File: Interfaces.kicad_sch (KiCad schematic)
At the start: 15 parts, among them J14 I2C1_Headers, J15 SPI1_Headers, J16 General_Pin_Header, J3 LPUART1_Headers, J8 Debug_Pins

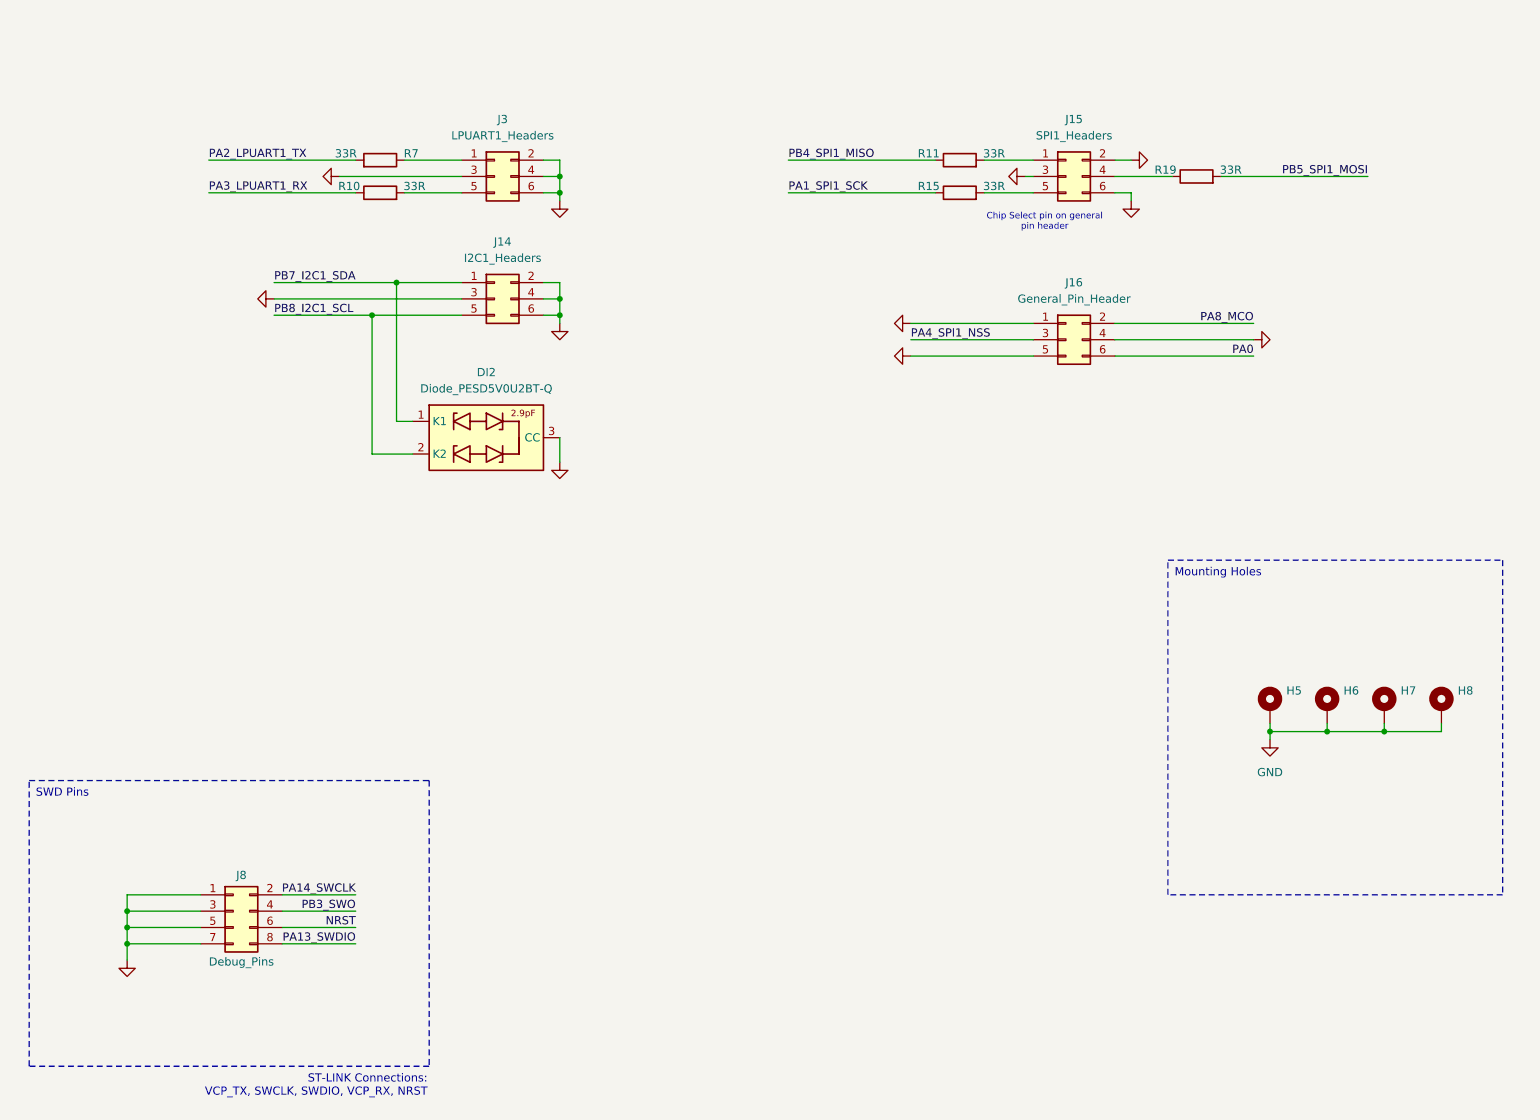
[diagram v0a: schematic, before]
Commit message: Update
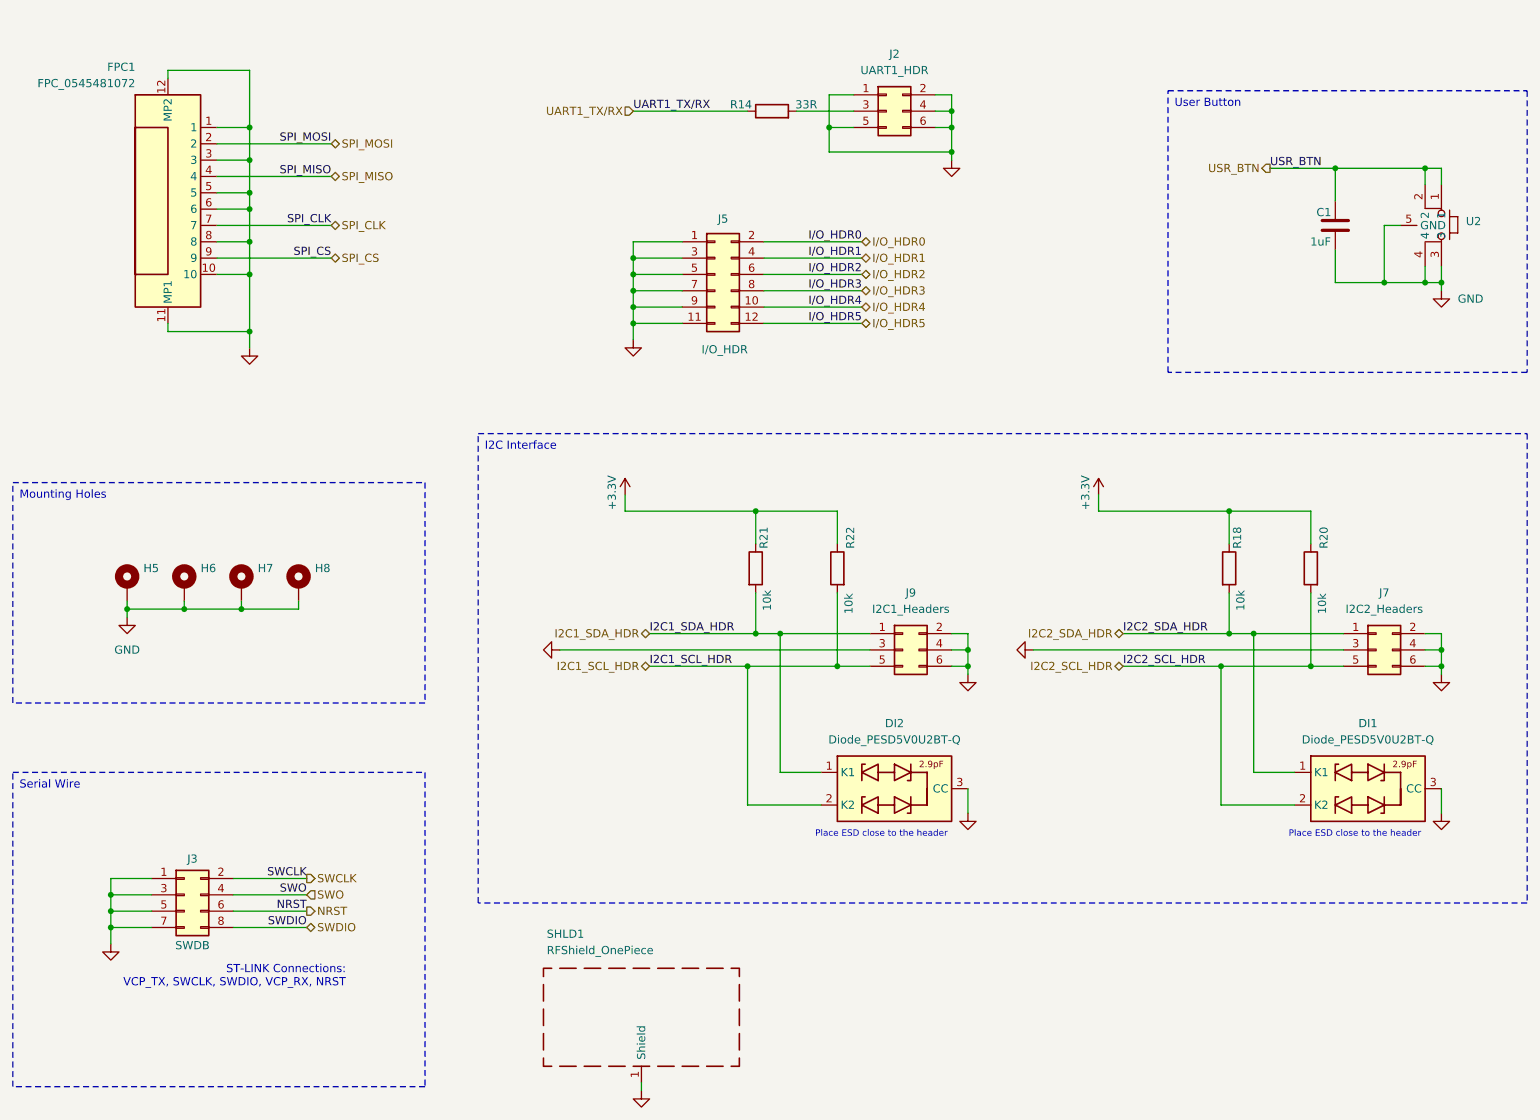
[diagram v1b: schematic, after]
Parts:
- removed J14: I2C1_Headers, Connector_PinHeader_2.54mm:PinHeader_2x03_P2.54mm_Horizontal, symbol Connector_Generic:Conn_02x03_Odd_Even
- removed J15: SPI1_Headers, Connector_PinHeader_2.54mm:PinHeader_2x03_P2.54mm_Horizontal, symbol Connector_Generic:Conn_02x03_Odd_Even
- removed J16: General_Pin_Header, Connector_PinHeader_2.54mm:PinHeader_2x03_P2.54mm_Horizontal, symbol Connector_Generic:Conn_02x03_Odd_Even
- removed J3: LPUART1_Headers, Connector_PinHeader_2.54mm:PinHeader_2x03_P2.54mm_Horizontal, symbol Connector_Generic:Conn_02x03_Odd_Even
- removed J8: Debug_Pins, Connector_PinHeader_2.54mm:PinHeader_2x04_P2.54mm_Horizontal, symbol Connector_Generic:Conn_02x04_Odd_Even
- removed R10, R11, R15, R19, R7: 33R, Resistor_SMD:R_0805_2012Metric, symbol Device:R
- added C1: 1uF, Capacitor_SMD:C_0805_2012Metric, symbol Device:C
- added DI1: Diode_PESD5V0U2BT-Q, Package_TO_SOT_SMD:SOT-23, symbol Personal_Projects:Diode_PESD5V0U2BT-Q
- added FPC1: FPC_0545481072, Personal_Project:FPC_0545481072, symbol Personal_Projects:FPC_0545481072
- added J2: UART1_HDR, Connector_PinHeader_2.54mm:PinHeader_2x03_P2.54mm_Horizontal, symbol Connector_Generic:Conn_02x03_Odd_Even
- added J3: SWDB, Connector_PinHeader_2.54mm:PinHeader_2x04_P2.54mm_Horizontal, symbol Connector_Generic:Conn_02x04_Odd_Even
- added J5: I/O_HDR, symbol Connector_Generic:Conn_02x06_Odd_Even
- added J7: I2C2_Headers, Connector_PinHeader_2.54mm:PinHeader_2x03_P2.54mm_Horizontal, symbol Connector_Generic:Conn_02x03_Odd_Even
- added J9: I2C1_Headers, Connector_PinHeader_2.54mm:PinHeader_2x03_P2.54mm_Horizontal, symbol Connector_Generic:Conn_02x03_Odd_Even
- added R14: 33R, Resistor_SMD:R_0805_2012Metric, symbol Device:R
- added R18, R20, R21, R22: 10k, Resistor_SMD:R_0805_2012Metric, symbol Device:R
- added SHLD1: RFShield_OnePiece, Personal_Project:RF_Shield_MS631-10F, symbol Device:RFShield_OnePiece
- added U2: ~, Personal_Project:Button_KMR231GLFS, symbol Personal_Projects:Button_KMR231GLFS
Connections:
- net GND: now also C1.1, DI1.3 (CC), FPC1.1, FPC1.10, FPC1.11 (MP1), FPC1.12 (MP2), FPC1.3, FPC1.5, FPC1.6, FPC1.8, J2.1 (Pin_1), J2.2 (Pin_2), J2.4 (Pin_4), J2.5 (Pin_5), J2.6 (Pin_6), J3.1 (Pin_1), J3.3 (Pin_3), J3.5 (Pin_5), J3.7 (Pin_7), J5.1 (Pin_1), J5.11 (Pin_11), J5.3 (Pin_3), J5.5 (Pin_5), J5.7 (Pin_7), J5.9 (Pin_9), J7.2 (Pin_2), J7.3 (Pin_3), J7.4 (Pin_4), J7.6 (Pin_6), J9.2 (Pin_2), J9.3 (Pin_3), J9.4 (Pin_4), J9.6 (Pin_6), SHLD1.1 (Shield), U2.3, U2.4, U2.5 (GND)
- net NRST: now also J3.6 (Pin_6)
- net PB7_I2C1_SDA renamed I2C1_SDA_HDR
- net I2C1_SDA_HDR: now also J9.1 (Pin_1), R21.2
- net PB8_I2C1_SCL renamed I2C1_SCL_HDR
- net I2C1_SCL_HDR: now also J9.5 (Pin_5), R22.2
- new net: J2.3 (Pin_3), R14.2
- new net +3.3V: R18.1, R20.1, R21.1, R22.1
- new net I2C2_SCL_HDR: DI1.2 (K2), J7.5 (Pin_5), R20.2
- new net I2C2_SDA_HDR: DI1.1 (K1), J7.1 (Pin_1), R18.2
- new net I/O_HDR0: J5.2 (Pin_2)
- new net I/O_HDR1: J5.4 (Pin_4)
- new net I/O_HDR2: J5.6 (Pin_6)
- new net I/O_HDR3: J5.8 (Pin_8)
- new net I/O_HDR4: J5.10 (Pin_10)
- new net I/O_HDR5: J5.12 (Pin_12)
- new net SPI_CLK: FPC1.7
- new net SPI_CS: FPC1.9
- new net SPI_MISO: FPC1.4
- new net SPI_MOSI: FPC1.2
- new net SWCLK: J3.2 (Pin_2)
- new net SWDIO: J3.8 (Pin_8)
- new net SWO: J3.4 (Pin_4)
- new net UART1_TX/RX: R14.1
- new net USR_BTN: C1.2, U2.1, U2.2
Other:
- note added: "Place ESD close to the header"
- note removed: "Chip Select pin on general pin header"
- moved on the sheet: H5, H6, H7, H8

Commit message: Update
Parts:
- J5: footprint (none) -> Connector_PinHeader_2.54mm:PinHeader_2x06_P2.54mm_Vertical
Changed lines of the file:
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@@
 			)
 		)
-		(property "Footprint" ""
+		(property "Footprint" "Connector_PinHeader_2.54mm:PinHeader_2x06_P2.54mm_Vertical"
 			(at 133.35 66.04 0)
 			(effects

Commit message: Update
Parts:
- J5: footprint Connector_PinHeader_2.54mm:PinHeader_2x06_P2.54mm_Vertical -> Connector_PinHeader_2.54mm:PinHeader_2x06_P2.54mm_Horizontal
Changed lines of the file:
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@@
 			)
 		)
-		(property "Footprint" "Connector_PinHeader_2.54mm:PinHeader_2x06_P2.54mm_Vertical"
+		(property "Footprint" "Connector_PinHeader_2.54mm:PinHeader_2x06_P2.54mm_Horizontal"
 			(at 133.35 66.04 0)
 			(effects

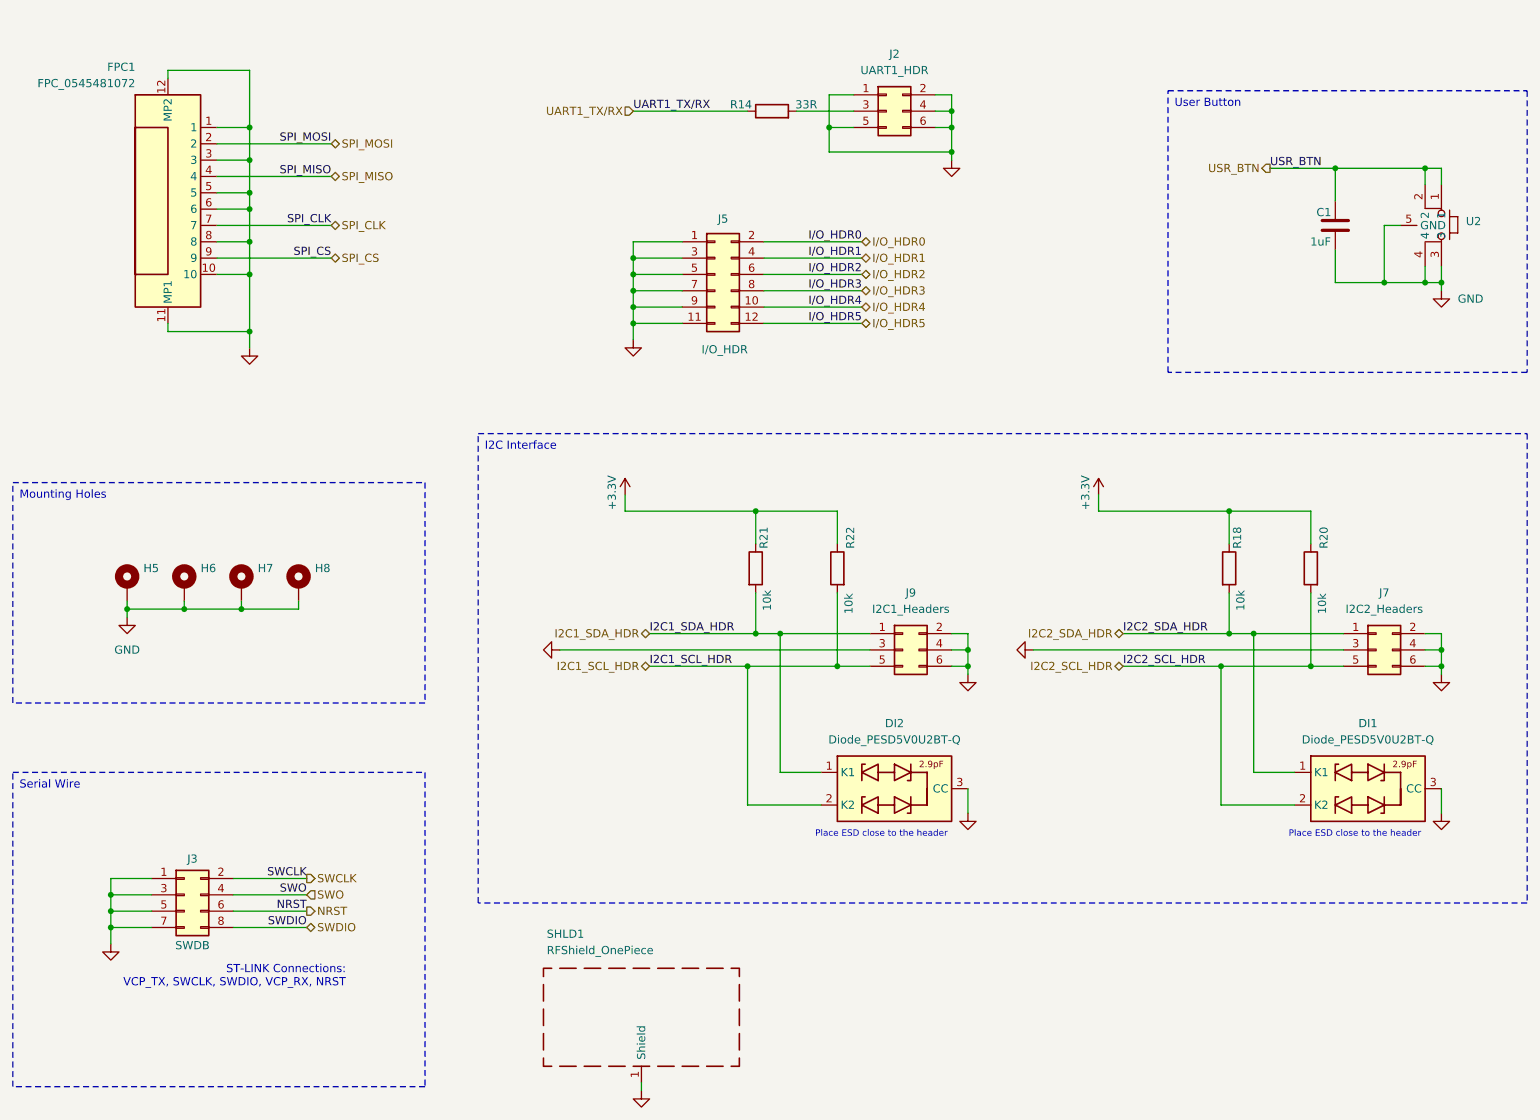
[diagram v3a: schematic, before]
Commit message: Update
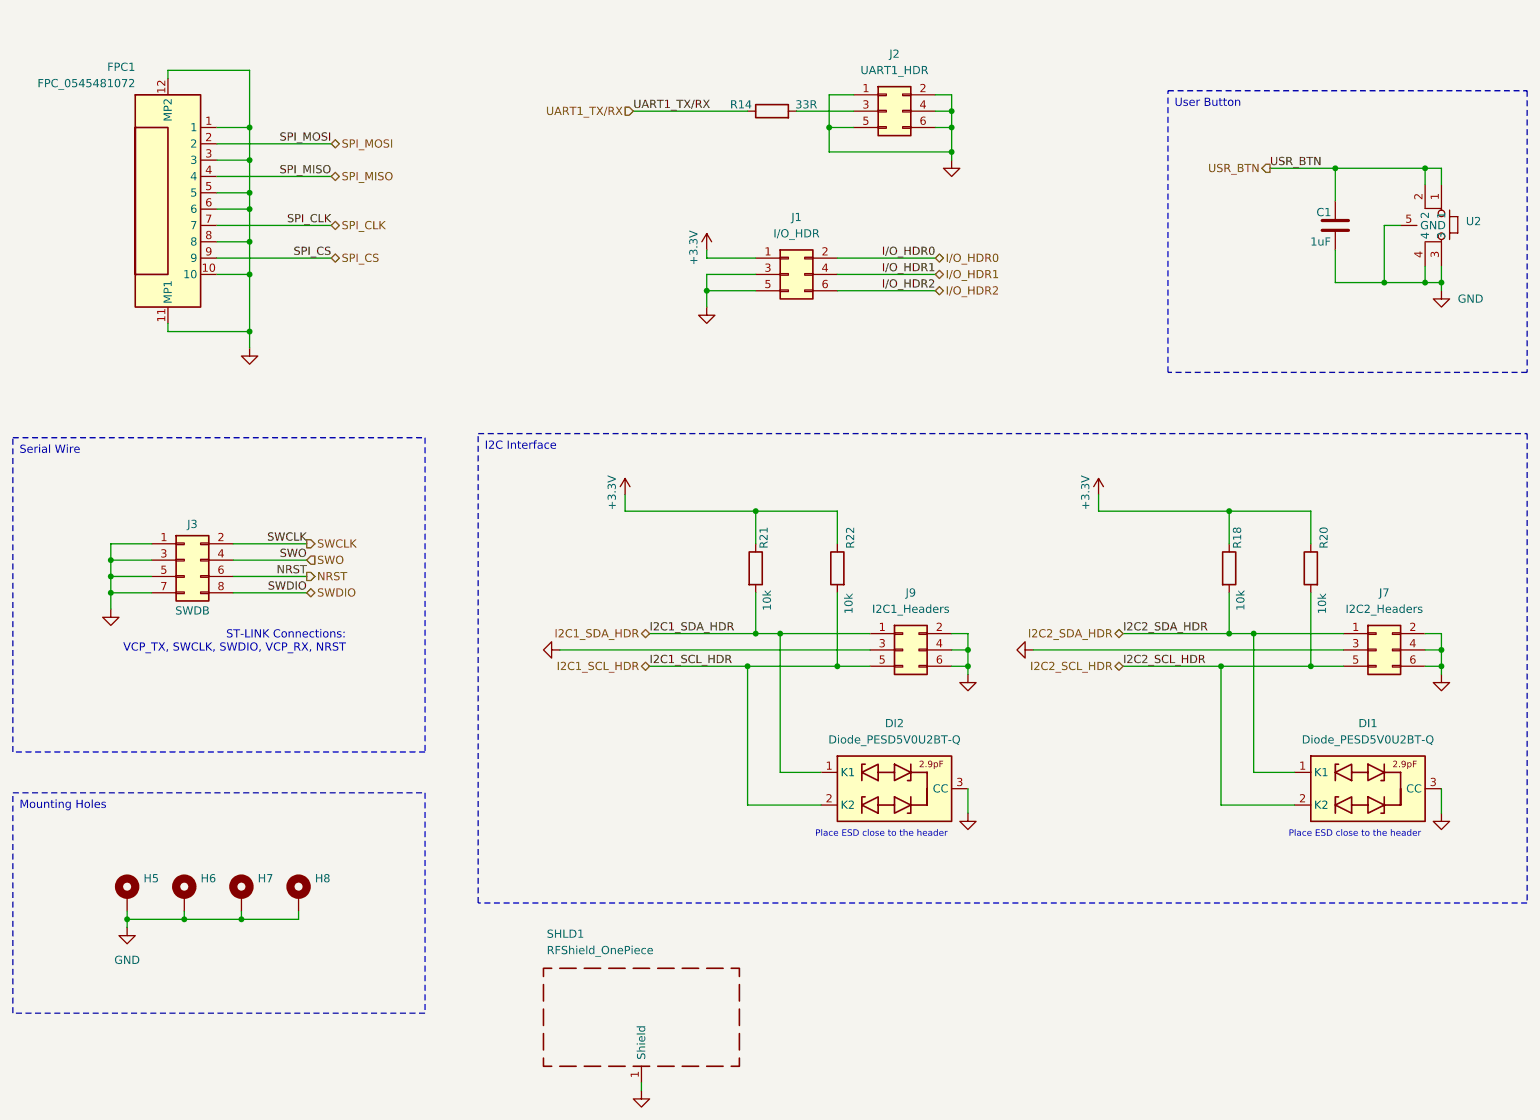
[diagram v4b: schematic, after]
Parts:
- removed J5: I/O_HDR, Connector_PinHeader_2.54mm:PinHeader_2x06_P2.54mm_Horizontal, symbol Connector_Generic:Conn_02x06_Odd_Even
- added J1: I/O_HDR, Connector_PinHeader_2.54mm:PinHeader_2x03_P2.54mm_Horizontal, symbol Connector_Generic:Conn_02x03_Odd_Even
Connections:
- net +3.3V: now also J1.1 (Pin_1)
- net GND: now also J1.3 (Pin_3), J1.5 (Pin_5)
- net I/O_HDR0: now also J1.2 (Pin_2)
- net I/O_HDR1: now also J1.4 (Pin_4)
- net I/O_HDR2: now also J1.6 (Pin_6)
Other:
- moved on the sheet: H5, H6, H7, H8, J3
